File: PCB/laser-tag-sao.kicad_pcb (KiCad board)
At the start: 2 copper layers, 99.8 x 43.6 mm, 18 parts, among them J1 SAO Connector, Q1 PN2222A, SW1 SW_Push, SW2 SW_Push, U1 ATTINY84A-PU, U2 TSOP38438, U3 OLED_0.91_128x32

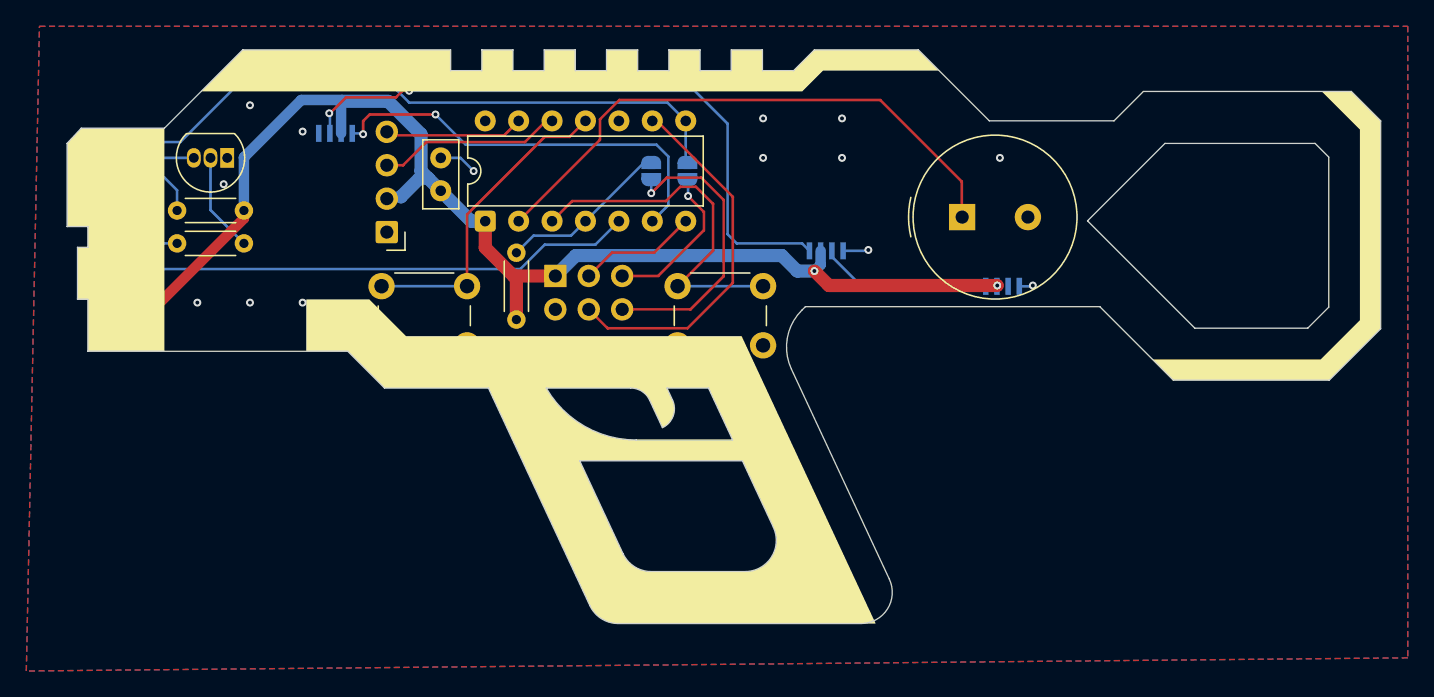
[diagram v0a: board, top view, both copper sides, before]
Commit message: adding silkscreen
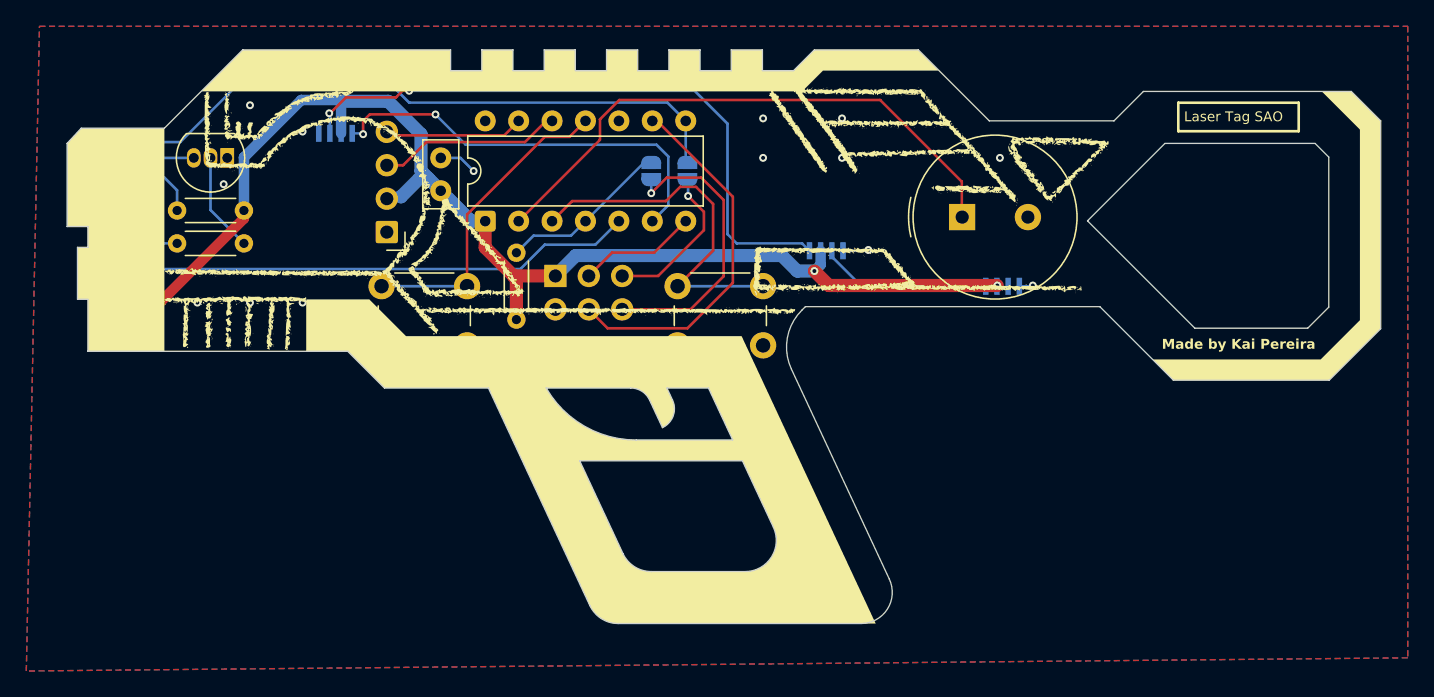
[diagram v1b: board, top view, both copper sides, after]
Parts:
- added G***: LOGO, LOGO, F.Cu at (208.1, 81.4)
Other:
- board text added: "Laser Tag SAO"
- board text added: "Made by Kai Pereira"
